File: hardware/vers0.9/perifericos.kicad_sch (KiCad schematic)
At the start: 7 parts, among them J4 Conn_02x13_Odd_Even, U7 74HC244, U8 74HC374

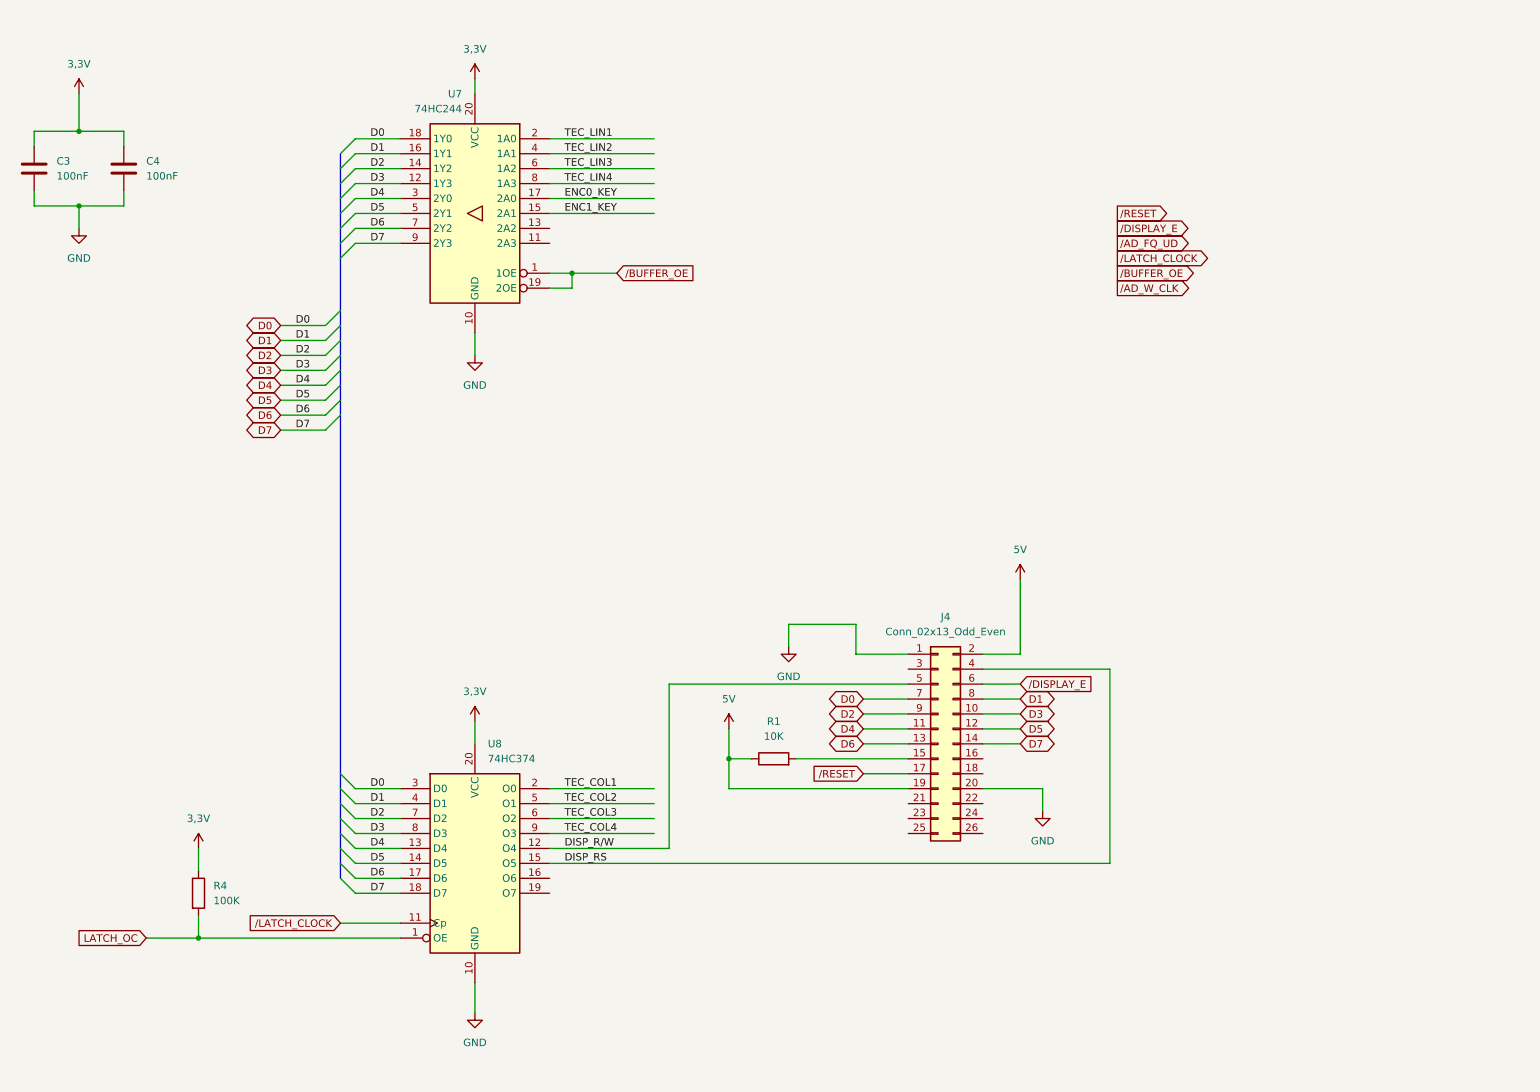
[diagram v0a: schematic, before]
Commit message: 250330-0836
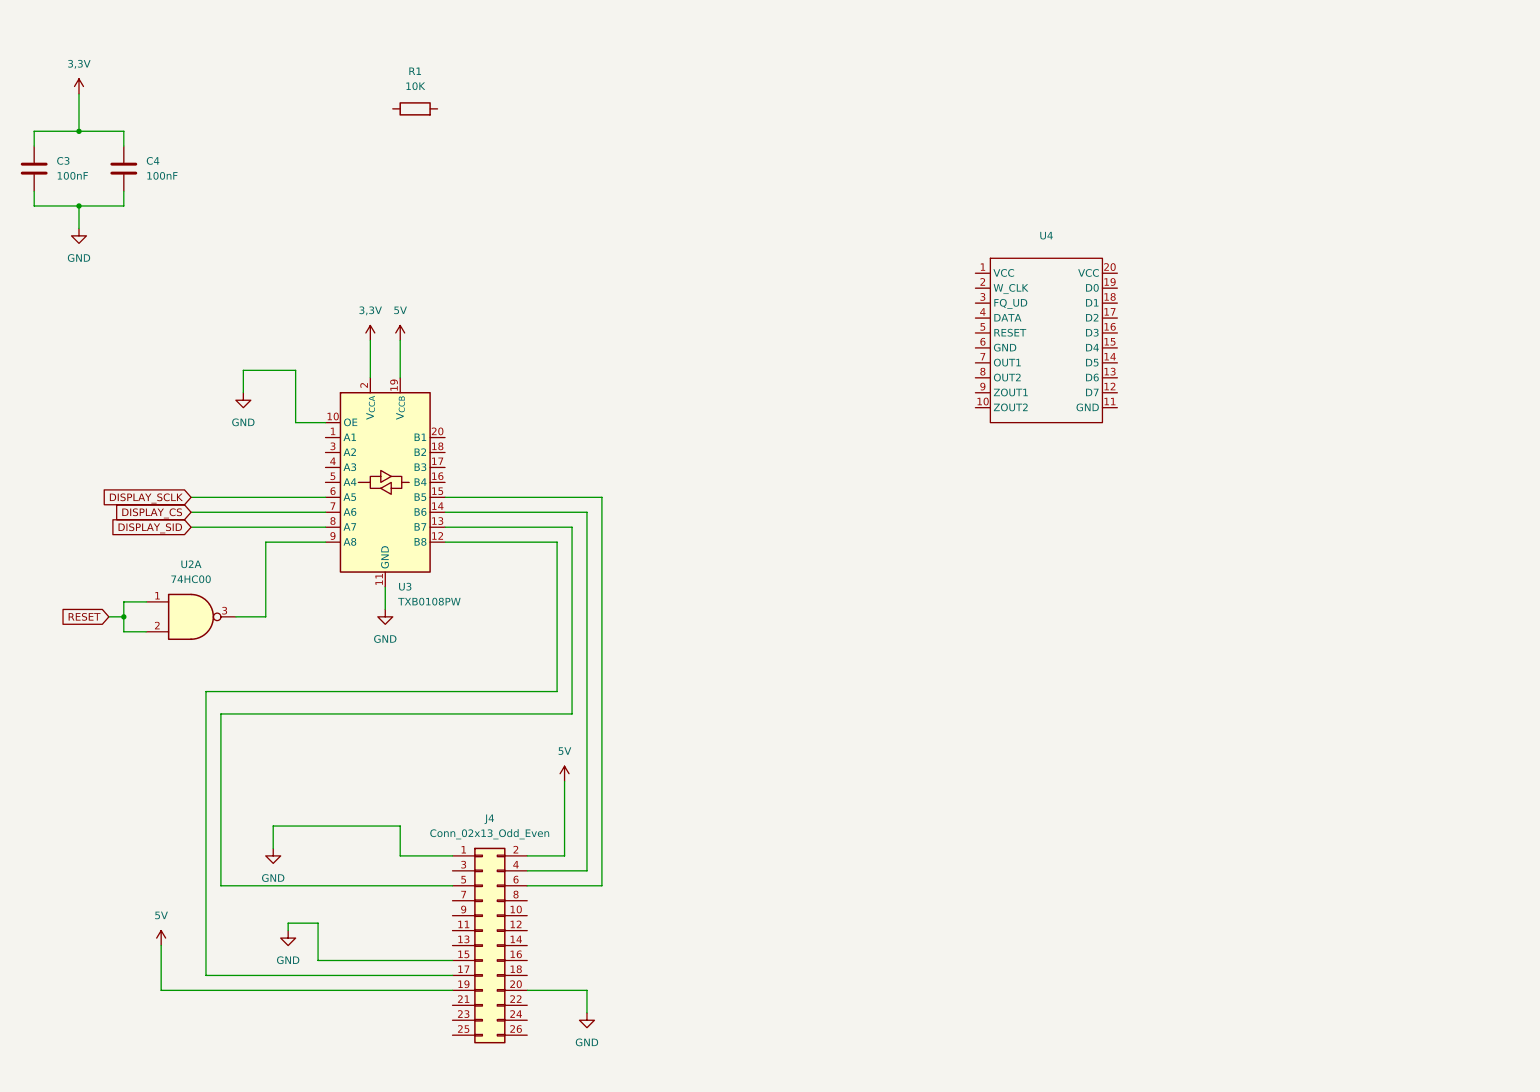
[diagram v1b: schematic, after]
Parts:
- removed R4: 100K, symbol Device:R
- removed U7: 74HC244, symbol 74xx:74HC244
- removed U8: 74HC374, symbol 74xx:74HC374
- added U2: 74HC00, symbol 74xx:74HC00
- added U3: TXB0108PW, Package_SO:TSSOP-20_4.4x6.5mm_P0.65mm, symbol Logic_LevelTranslator:TXB0108PW
- added U4: ~, symbol dev_boards:HC-SR08
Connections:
- net 3,3V: now also U3.2 (V_{CCA})
- net 5V: now also U3.19 (V_{CCB}); no longer R1.1
- net GND: now also J4.15 (Pin_15), U3.10 (OE), U3.11 (GND)
- net at R1.2: no longer J4.15 (Pin_15)
- net D0: no longer names the net of J4.7 (Pin_7)
- net D1: no longer names the net of J4.8 (Pin_8)
- net D2: no longer names the net of J4.9 (Pin_9)
- net D3: no longer names the net of J4.10 (Pin_10)
- net D4: no longer names the net of J4.11 (Pin_11)
- net D5: no longer names the net of J4.12 (Pin_12)
- net D6: no longer names the net of J4.13 (Pin_13)
- net D7: no longer names the net of J4.14 (Pin_14)
- net DISP_RS: no longer names the net of J4.4 (Pin_4)
- net DISP_RS: now also U3.14 (B6)
- net DISP_R/W: no longer names the net of J4.5 (Pin_5)
- net DISP_R/W: now also U3.13 (B7)
- net /DISPLAY_E: no longer names the net of J4.6 (Pin_6)
- net /DISPLAY_E: now also U3.15 (B5)
- net /RESET: no longer names the net of J4.17 (Pin_17)
- net /RESET: now also U3.12 (B8)
- new net: U2.3, U3.9 (A8)
- new net DISPLAY_CS: U3.7 (A6)
- new net DISPLAY_SCLK: U3.6 (A5)
- new net DISPLAY_SID: U3.8 (A7)
- new net RESET: U2.1, U2.2
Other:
- moved on the sheet: J4, R1

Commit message: 250404-0705
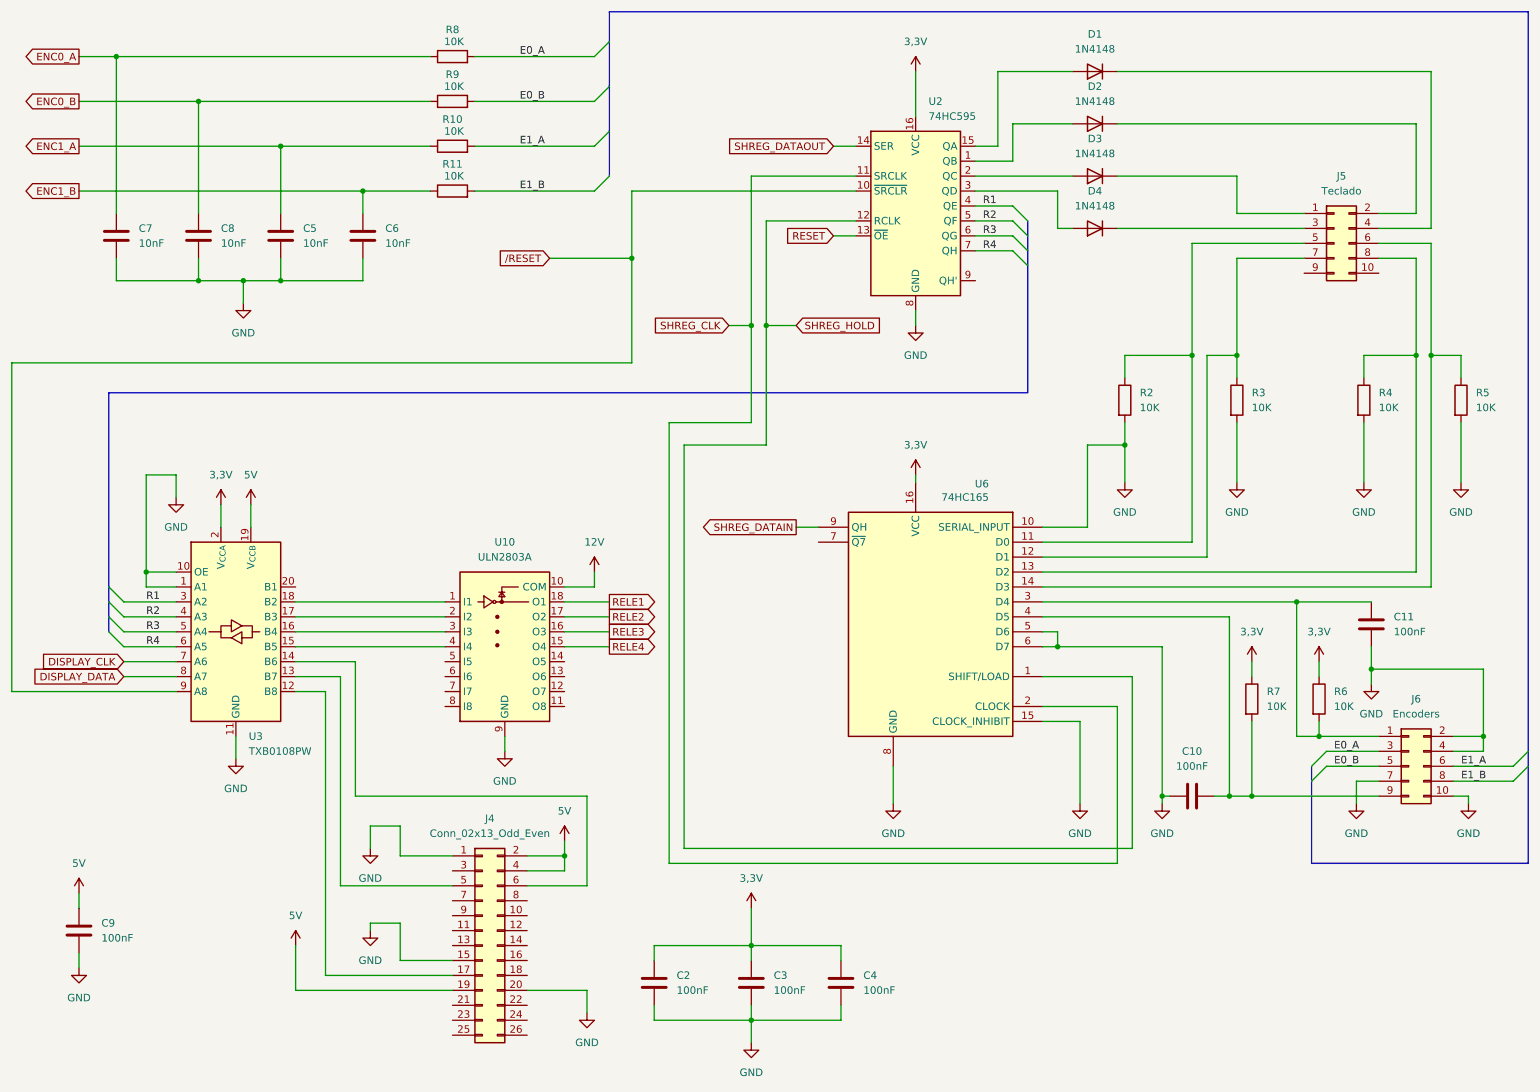
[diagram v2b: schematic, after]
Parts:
- removed R1: 10K, symbol Device:R
- removed U2: 74HC00, symbol 74xx:74HC00
- removed U4: ~, symbol dev_boards:HC-SR08
- added C10, C11, C2, C9: 100nF, symbol Device:C
- added C5, C6, C7, C8: 10nF, symbol Device:C
- added D1, D2, D3, D4: 1N4148, Diode_THT:D_DO-35_SOD27_P7.62mm_Horizontal, symbol Diode:1N4148
- added J5: Teclado, symbol Connector_Generic:Conn_02x05_Odd_Even
- added J6: Encoders, symbol Connector_Generic:Conn_02x05_Odd_Even
- added R10, R11, R2, R3, R4, R5, R6, R7, R8, R9: 10K, symbol Device:R
- added U10: ULN2803A, symbol Transistor_Array:ULN2803A
- added U2: 74HC595, symbol 74xx:74HC595
- added U6: 74HC165, symbol 74xx:74HC165
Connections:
- net 3,3V: now also C2.1, R6.1, R7.1, U2.16 (VCC), U6.16 (VCC)
- net 5V: now also J4.4 (Pin_4), C9.1
- net GND: now also U3.1 (A1), C10.1, C11.2, C2.2, C5.2, C6.2, C7.2, C8.2, C9.2, J6.10 (Pin_10), J6.2 (Pin_2), J6.4 (Pin_4), J6.7 (Pin_7), R2.2, R3.2, R4.2, R5.2, U10.9 (GND), U2.8 (GND), U6.10 (SERIAL_INPUT), U6.15 (CLOCK_INHIBIT), U6.5 (D6), U6.6 (D7), U6.8 (GND)
- net RESET: now also U2.13 (~{OE})
- net at U3.14 (B6): now also J4.6 (Pin_6); no longer J4.4 (Pin_4)
- net at U3.15 (B5): now also U10.4 (I4); no longer J4.6 (Pin_6)
- net at U3.16 (B4): now also U10.3 (I3)
- net at U3.17 (B3): now also U10.2 (I2)
- net at U3.18 (B2): now also U10.1 (I1)
- net R1: now reaches U3.3 (A2)
- net R1: now also U2.4 (QE)
- net R2: now reaches U3.4 (A3)
- net R2: now also U2.5 (QF)
- net R3: now reaches U3.5 (A4)
- net R3: now also U2.6 (QG)
- net /RESET: now reaches U3.9 (A8)
- net /RESET: now also U2.10 (~{SRCLR})
- net DISPLAY_CS renamed DISPLAY_CLK
- net DISPLAY_SCLK renamed R4
- net R4: now also U2.7 (QH)
- net DISPLAY_SID renamed DISPLAY_DATA
- new net: J5.5 (Pin_5), R2.1, U6.11 (D0)
- new net: J5.7 (Pin_7), R3.1, U6.12 (D1)
- new net: J5.8 (Pin_8), R4.1, U6.13 (D2)
- new net: J5.6 (Pin_6), R5.1, U6.14 (D3)
- new net: C11.1, J6.1 (Pin_1), R6.2, U6.3 (D4)
- new net: C10.2, J6.9 (Pin_9), R7.2, U6.4 (D5)
- new net: D1.1 (K), J5.4 (Pin_4)
- new net: D1.2 (A), U2.15 (QA)
- new net: D3.1 (K), J5.1 (Pin_1)
- new net: D3.2 (A), U2.2 (QC)
- new net: D2.2 (A), U2.1 (QB)
- new net: D4.2 (A), U2.3 (QD)
- new net: D4.1 (K), J5.3 (Pin_3)
- new net: D2.1 (K), J5.2 (Pin_2)
- new net 12V: U10.10 (COM)
- new net E0_A: J6.3 (Pin_3), R8.2
- new net E0_B: J6.5 (Pin_5), R9.2
- new net E1_A: J6.6 (Pin_6), R10.2
- new net E1_B: J6.8 (Pin_8), R11.2
- new net ENC0_A: C7.1, R8.1
- new net ENC0_B: C8.1, R9.1
- new net ENC1_A: C5.1, R10.1
- new net ENC1_B: C6.1, R11.1
- new net RELE1: U10.18 (O1)
- new net RELE2: U10.17 (O2)
- new net RELE3: U10.16 (O3)
- new net RELE4: U10.15 (O4)
- new net SHREG_CLK: U2.11 (SRCLK), U6.2 (CLOCK)
- new net SHREG_DATAIN: U6.9 (QH)
- new net SHREG_DATAOUT: U2.14 (SER)
- new net SHREG_HOLD: U2.12 (RCLK), U6.1 (SHIFT/LOAD)
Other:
- moved on the sheet: C3, C4, U3
